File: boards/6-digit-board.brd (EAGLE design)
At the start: 150 x 70 mm, 53 parts

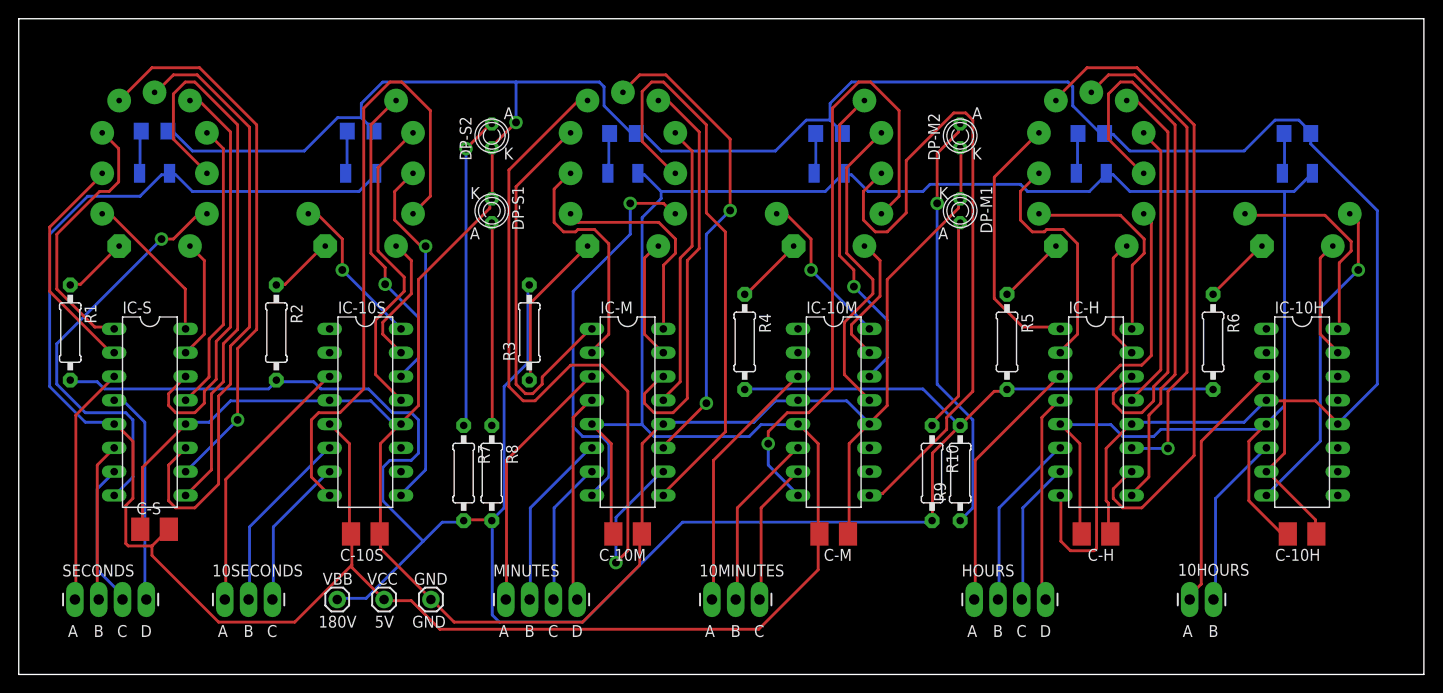
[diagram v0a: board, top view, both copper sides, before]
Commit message: put all the downloaded files into directories
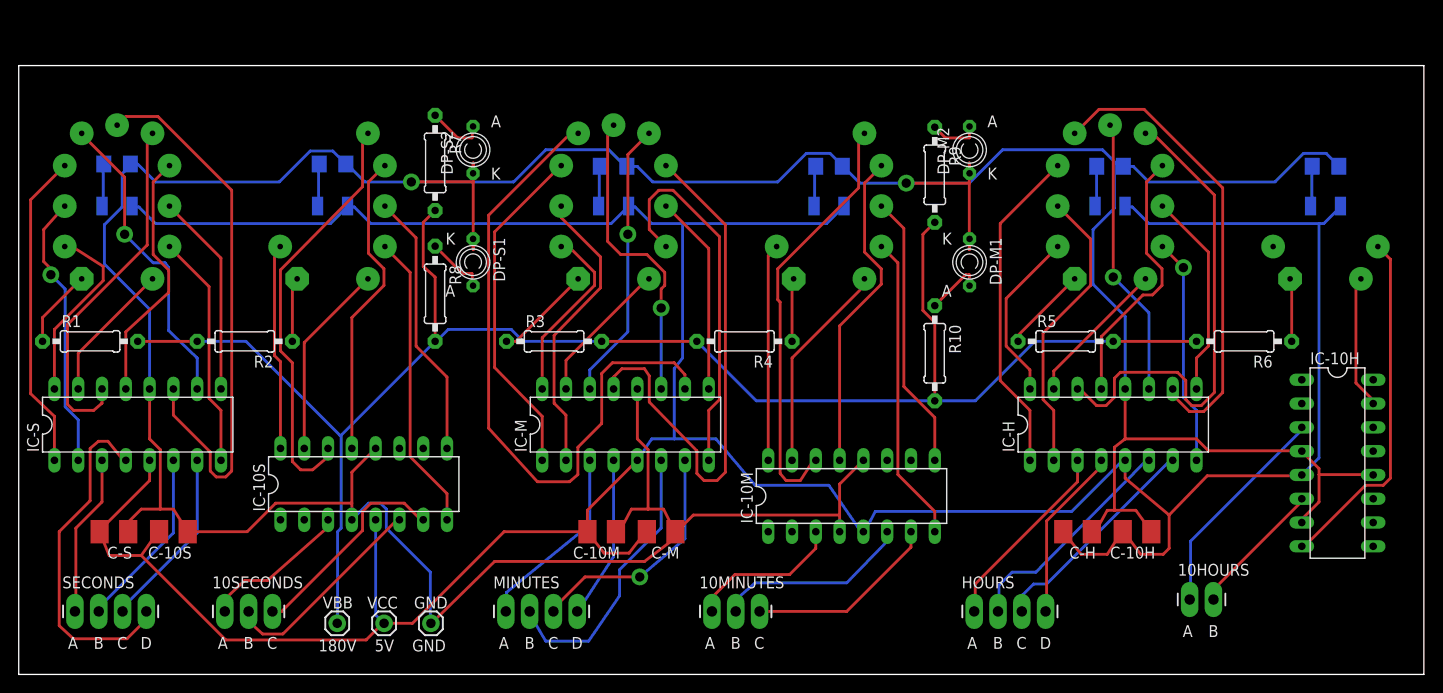
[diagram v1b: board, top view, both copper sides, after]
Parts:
- moved R7 33.3 mm to (44.5, 54.6)
- moved R9 32.0 mm to (97.8, 53.3), turned to 270 degrees
- moved C-10S 20.5 mm to (16.5, 15.2)
- moved R8 20.1 mm to (44.5, 40.6)
- moved C-M 18.4 mm to (68.6, 15.2)
- moved C-10H 17.6 mm to (119.4, 15.2)
- moved R10 12.8 mm to (97.8, 34.3)
- moved IC-10M 9.15 mm to (88.9, 19.1), turned to 0 degrees
- moved IC-10S 7.68 mm to (36.8, 20.3), turned to 0 degrees
- moved IC-10H 6.62 mm to (140.8, 22.6)
- moved R5 6.26 mm to (111.8, 35.6), turned to 0 degrees
- moved DP-S1 5.85 mm to (48.5, 44.0)
- moved DP-M1 5.59 mm to (101.5, 44.0)
- moved LED1 5.32 mm to (10.5, 50.0)
- moved R-L1 5.32 mm to (10.5, 54.5)
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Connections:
- removed net N$24: 10HOUR.0, IC-10H.16
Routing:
- net VCC: track 414.5 -> 366.0 mm
- net VBB: track 230.9 -> 183.1 mm
- net N$29: track 72.2 -> 29.5 mm
- net N$35: track 62.6 -> 21.4 mm
- net N$10: track 45.5 -> 5.38 mm, vias 1 -> 0
- net N$51: track 61.1 -> 21.8 mm
- net N$16: track 61.1 -> 22.1 mm
- net N$28: track 68.2 -> 32.8 mm, vias 1 -> 0
- net N$44: track 67.1 -> 31.9 mm
- net N$12: track 33.6 -> 6.16 mm, vias 1 -> 0
- net N$36: track 30.6 -> 57.4 mm
- net N$55: track 58.8 -> 33.1 mm
- net N$15: track 49.0 -> 24.3 mm, vias 0 -> 1
- net N$24: track 22.5 -> 0.00 mm
- net N$19: track 52.3 -> 29.9 mm
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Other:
- board size 150 x 70 mm -> 150 x 65 mm
